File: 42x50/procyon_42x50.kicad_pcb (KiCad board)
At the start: 4 copper layers, 42 x 49.6 mm, 34 parts, among them J1 Conn_01x07_Pin, Q1 AO3401A, U1 mXT336UD-MAU002

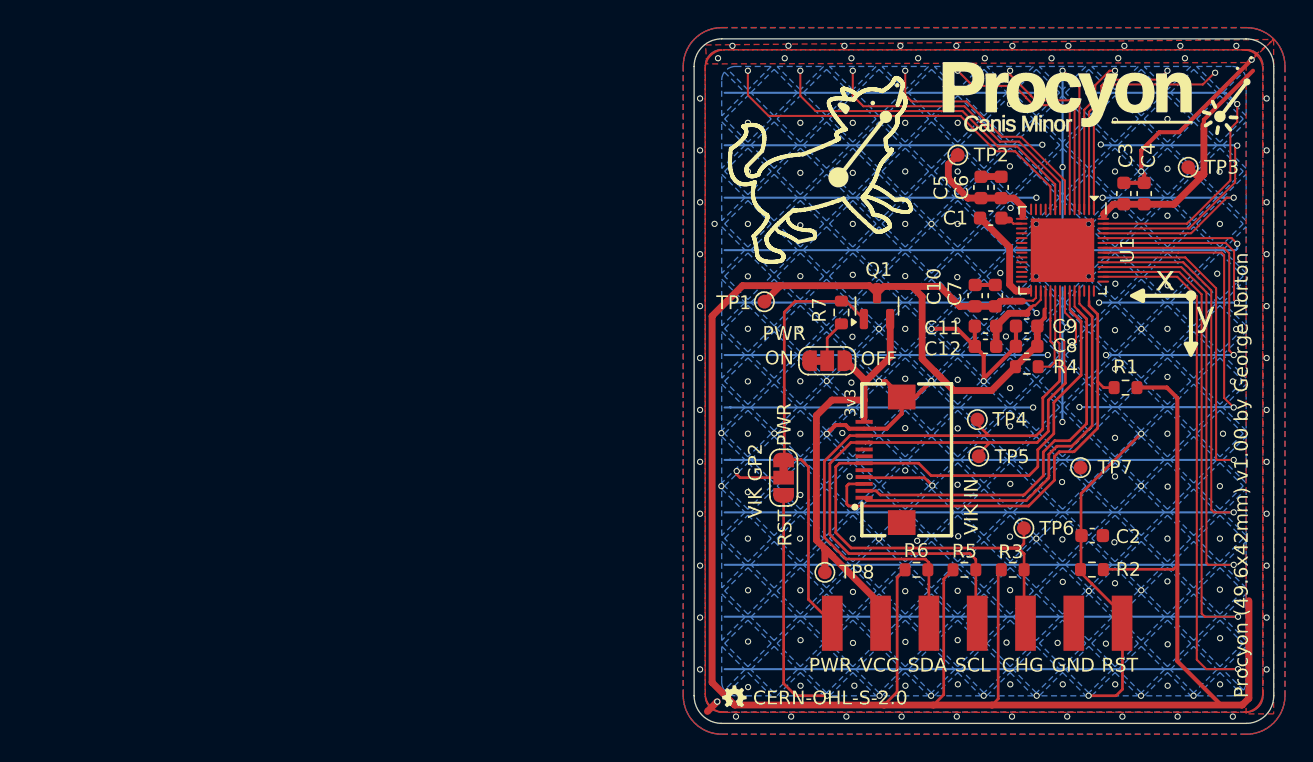
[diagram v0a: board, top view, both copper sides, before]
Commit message: silkscreen
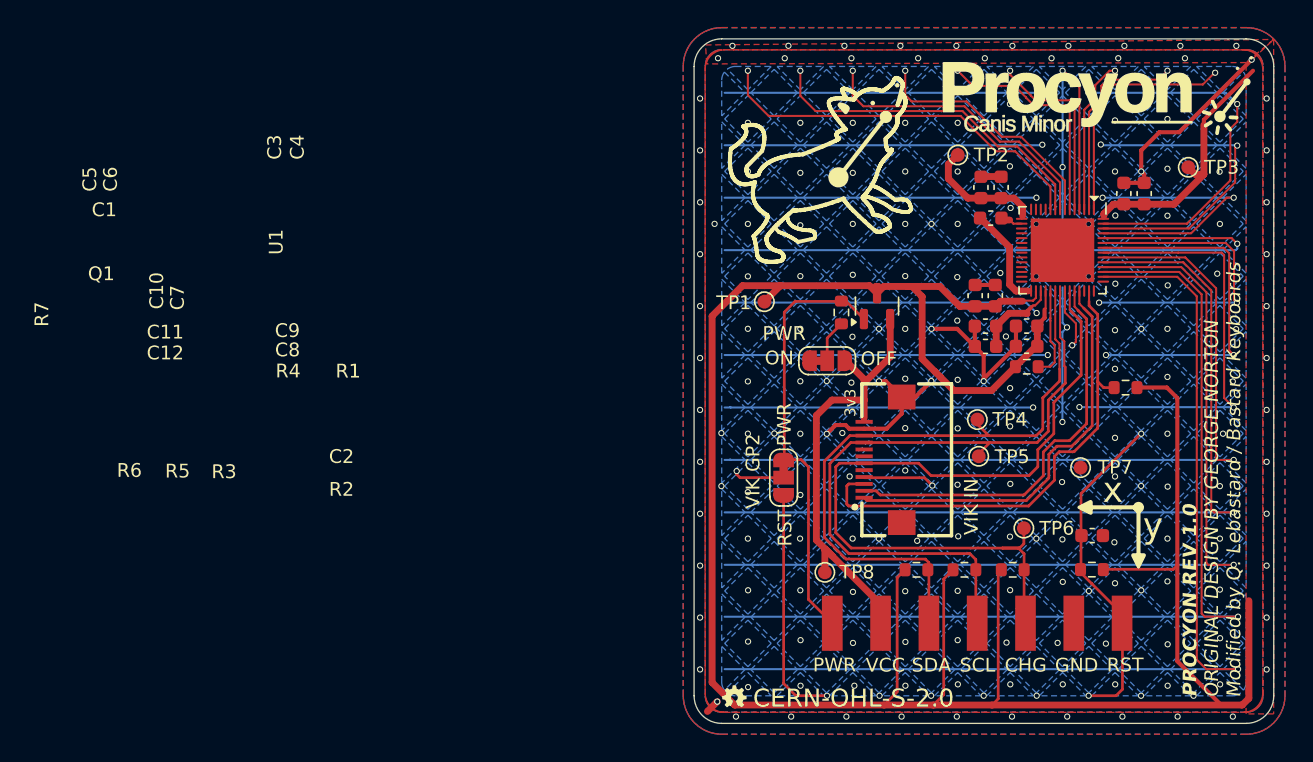
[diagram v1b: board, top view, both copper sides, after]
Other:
- board text added: "ORIGINAL DESIGN BY GEORGE NORTON Modified by Q. Lebastard / Bastard Keyboards"
- board text added: "PROCYON REV 1.0"
- board text removed: "Procyon (49.6x42mm) v1.00 by George Norton"
